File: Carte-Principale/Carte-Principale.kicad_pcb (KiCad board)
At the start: 2 copper layers, 140 x 118.1 mm, 108 parts, among them J1 Moteur_Gauche, J10 Sensors, J13 Encodeur_G, J15 AX12, J18 PCA9685, J2 GND, J21 I2C Screen, J3 12VA, J4 5V, J5 Moteur_Droit, J6 UART_Debug, J7 GPIO, J8 Encodeur_D, J9 SPI3, Q1 BC817, Q2 BSS138, Q3 BSS138, Q4 BSS138, Q5 BSS138, SW1 Rouge, SW2 Bleu, SW3 Jaune, SW4 Vert, U2 NUCLEOH723ZG, U3 AM26LV32xD, U4 74LVC1G3157, U5 74LVC1G3157, U6 74LVC1G3157, U7 74LVC1G3157

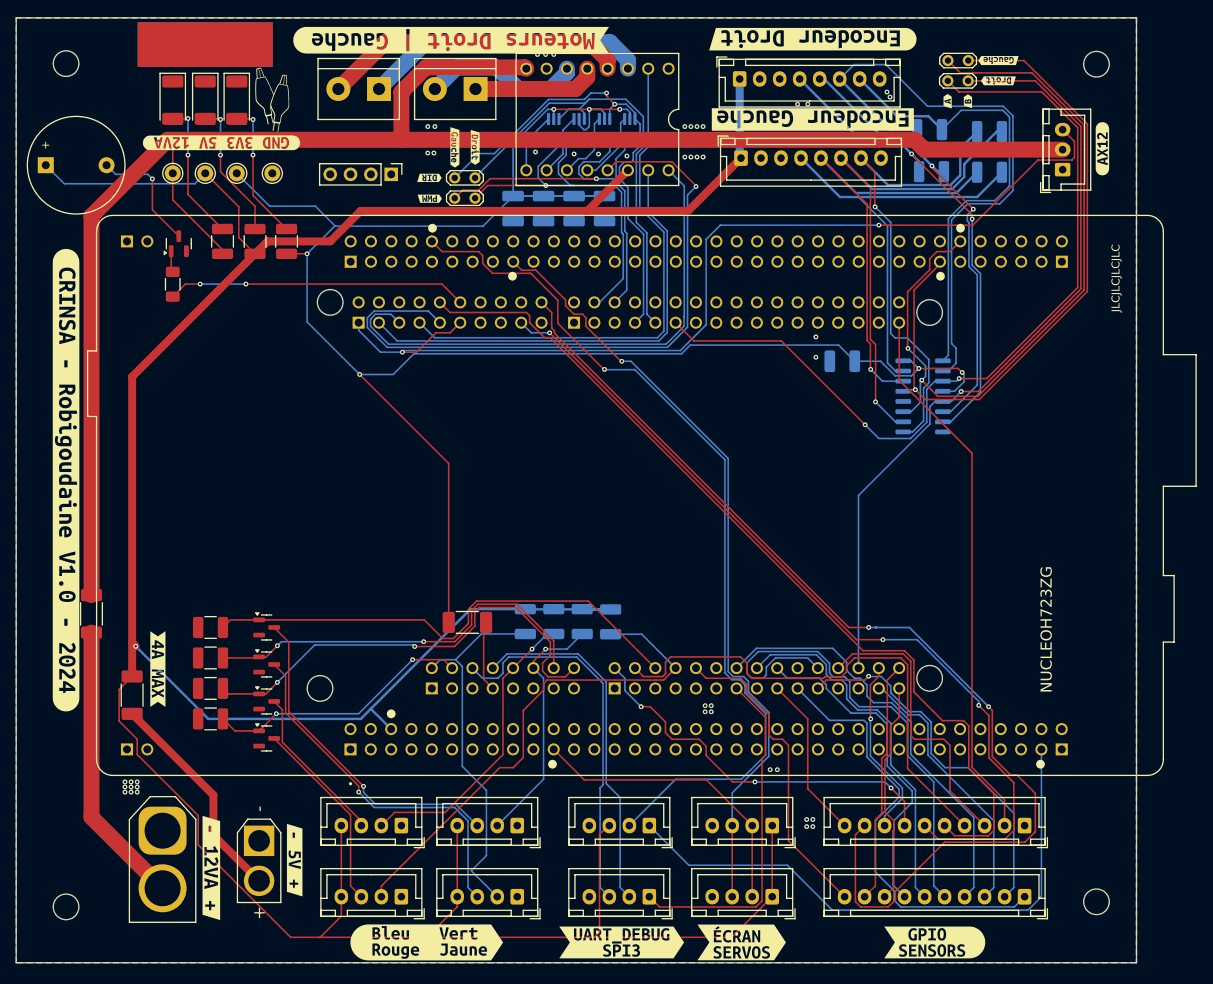
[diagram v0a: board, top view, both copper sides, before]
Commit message: abcdefgh
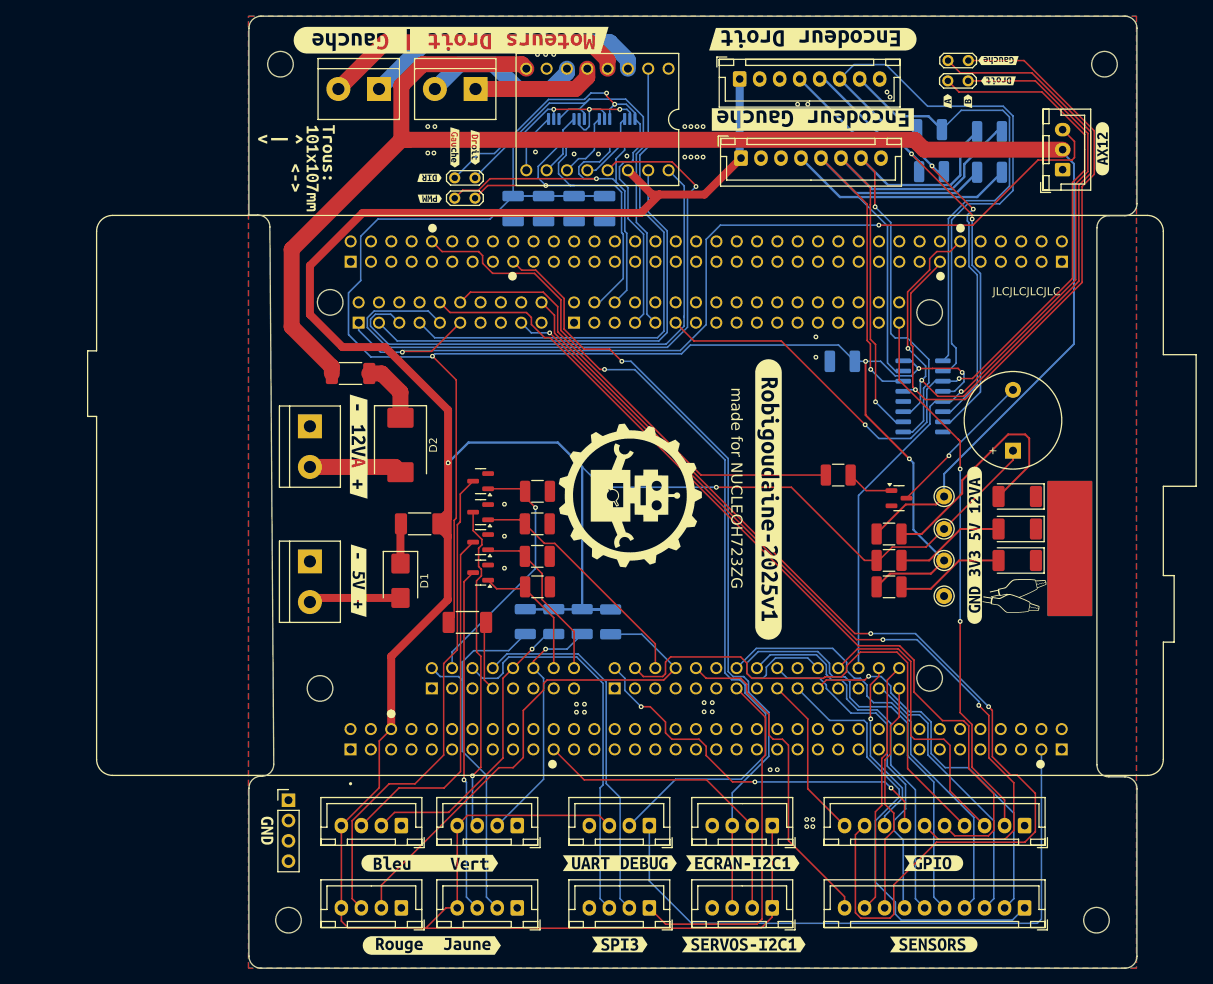
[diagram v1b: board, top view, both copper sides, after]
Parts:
- removed kibuzzard-2: G***, kibuzzard-66C478F6
- removed kibuzzard-5: G***, kibuzzard-66C08EFC
- removed kibuzzard-66F08110: G***, kibuzzard-66F08110
- removed kibuzzard-66FDA353: G***, kibuzzard-66FDA353
- removed kibuzzard-67547681: G***, kibuzzard-67547681
- removed kibuzzard-67548783: G***, kibuzzard-67548783
- removed kibuzzard-67548BCB: G***, kibuzzard-67548BCB
- added D1: D, Diode_SMD:D_SMB, F.Cu at (118.0, 99.6)
- added D2: 200V 3A, Diode_SMD:D_SMC, F.Cu at (118.0, 82.6)
- added kibuzzard-676C5963: G***, kibuzzard-676C5963, F.Cu at (164.0, 89.4)
- added kibuzzard-676C6030: G***, kibuzzard-676C6030, F.Cu at (124.3, 32.0)
- added kibuzzard-676EB23A: G***, kibuzzard-676EB23A, F.Cu at (121.9, 145.2)
- added kibuzzard-676EB26A: G***, kibuzzard-676EB26A, F.Cu at (121.7, 134.9)
- added kibuzzard-676EB29A: G***, kibuzzard-676EB29A, F.Cu at (145.4, 145.0)
- added kibuzzard-676EB2FD: G***, kibuzzard-676EB2FD, F.Cu at (160.9, 145.0)
- added kibuzzard-676EB30E: G***, kibuzzard-676EB30E, F.Cu at (184.7, 134.9)
- added kibuzzard-676EB31C: G***, kibuzzard-676EB31C, F.Cu at (184.7, 145.0)
- added kibuzzard-676EB336: G***, kibuzzard-676EB336, F.Cu at (145.4, 134.9)
- added kibuzzard-676EB35D: G***, kibuzzard-676EB35D, F.Cu at (160.8, 134.9)
- added kibuzzard-676EB466: G***, kibuzzard-676EB466, F.Cu at (105.0, 48.0)
- added kibuzzard-676FE8DD: G***, kibuzzard-676FE8DD, F.Cu at (101.3, 130.8)
- G1: moved to F.Cu
- J3: footprint Connector_AMASS:AMASS_XT60-M_1x02_P7.20mm_Vertical -> TerminalBlock:TerminalBlock_bornier-2_P5.08mm
- J4: footprint Connector_AMASS:AMASS_XT30U-M_1x02_P5.0mm_Vertical -> TerminalBlock:TerminalBlock_bornier-2_P5.08mm
- R2: footprint Resistor_SMD:R_1206_3216Metric_Pad1.30x1.75mm_HandSolder -> Resistor_SMD:R_1210_3225Metric_Pad1.30x2.65mm_HandSolder
- U2: value NUCLEOH723ZG -> made for NUCLEOH723ZG
- moved BZ1 126.1 mm to (194.6, 83.3), turned to 90 degrees
- moved D7 116.6 mm to (195.1, 89.0), turned to 180 degrees
- moved D5 114.8 mm to (195.1, 93.1), turned to 180 degrees
- moved D6 113.3 mm to (195.1, 97.0), turned to 180 degrees
- moved G*** 111.6 mm to (194.8, 101.5), turned to -90 degrees
- moved kibuzzard-66F08121 106.7 mm to (189.8, 95.1), turned to 90 degrees
- moved TP5 104.5 mm to (186.0, 89.0), turned to 180 degrees
- moved TP3 102.5 mm to (186.0, 93.1), turned to 180 degrees
- moved TP1 100.8 mm to (186.0, 97.0), turned to 180 degrees
- moved TP2 99.2 mm to (186.0, 101.5), turned to 180 degrees
- moved Q1 95.5 mm to (180.3, 89.2), turned to 0 degrees
- moved R4 91.0 mm to (179.1, 93.7), turned to 0 degrees
- moved R3 88.7 mm to (179.1, 97.0), turned to 0 degrees
- moved R1 86.8 mm to (179.1, 100.3), turned to 0 degrees
- moved R2 86.5 mm to (172.7, 86.4), turned to 0 degrees
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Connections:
- F1 pad 1: Net-(J3-Pin_2) -> Net-(D2-K)
- F2 pad 1: Net-(J4-Pin_2) -> Net-(D1-K)
- J3 pad 2: Net-(J3-Pin_2) -> Net-(D2-A)
- J4 pad 2: Net-(J4-Pin_2) -> Net-(D1-A)
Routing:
- net Net-(Q5-D): track 24.3 -> 62.0 mm
- net /PG3: track 57.4 -> 21.5 mm, vias 2 -> 0
- net Net-(J3-Pin_2): track 35.6 -> 0.00 mm
- net /PG2: track 50.5 -> 16.8 mm, vias 2 -> 0
- net /PD5: track 61.9 -> 30.4 mm
- net Net-(J4-Pin_2): track 27.5 -> 0.00 mm
- net Net-(Q4-D): track 20.0 -> 44.5 mm
- net /PA6: track 37.5 -> 57.5 mm, vias 2 -> 0
- net +5V: track 418.8 -> 401.2 mm, vias 1 -> 2
- net Net-(D7-A): track 17.6 -> 31.2 mm, vias 2 -> 0
- net Net-(D2-A): track 0.00 -> 11.6 mm
- net Net-(D1-A): track 0.00 -> 10.7 mm
- net +3.3V: track 240.8 -> 250.5 mm, vias 7 -> 8
- net +12VA: track 213.3 -> 204.9 mm
- net Net-(D2-K): track 0.00 -> 7.07 mm
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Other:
- board size 140 x 118.1 mm -> 111 x 119 mm
- board text added: "JP6 OFF & SB7 ON pour PB13 !"
